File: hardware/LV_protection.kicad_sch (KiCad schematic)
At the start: 4 parts, among them J2 Conn_01x02, Q2 NMOS

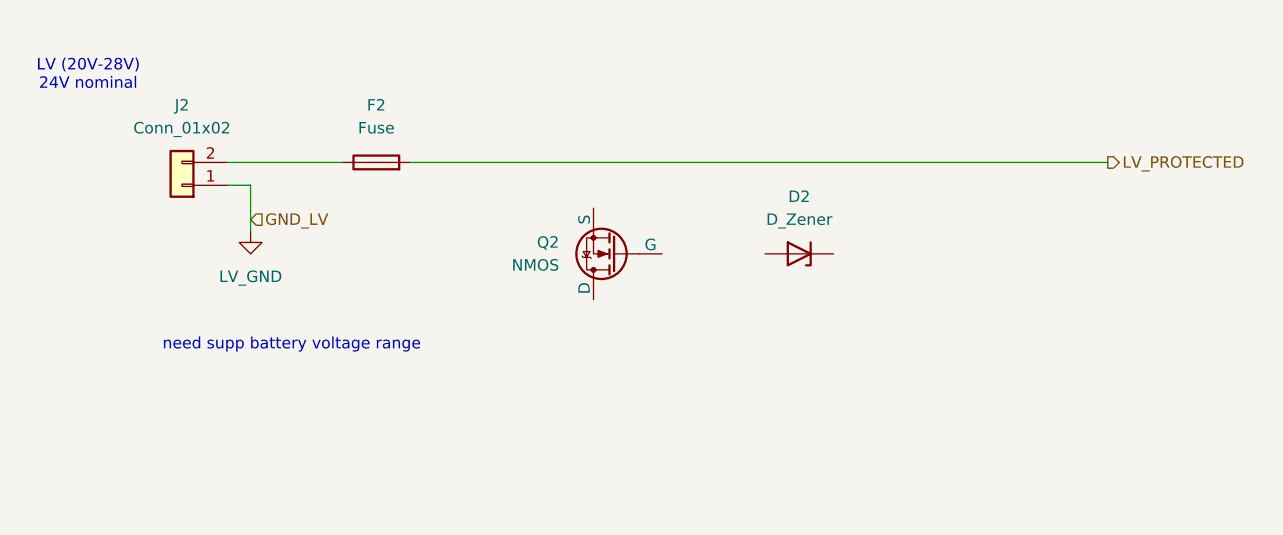
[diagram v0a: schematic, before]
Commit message: did fan circuits, added MCU design block, made buck converter, added VIP sensing + soft start?
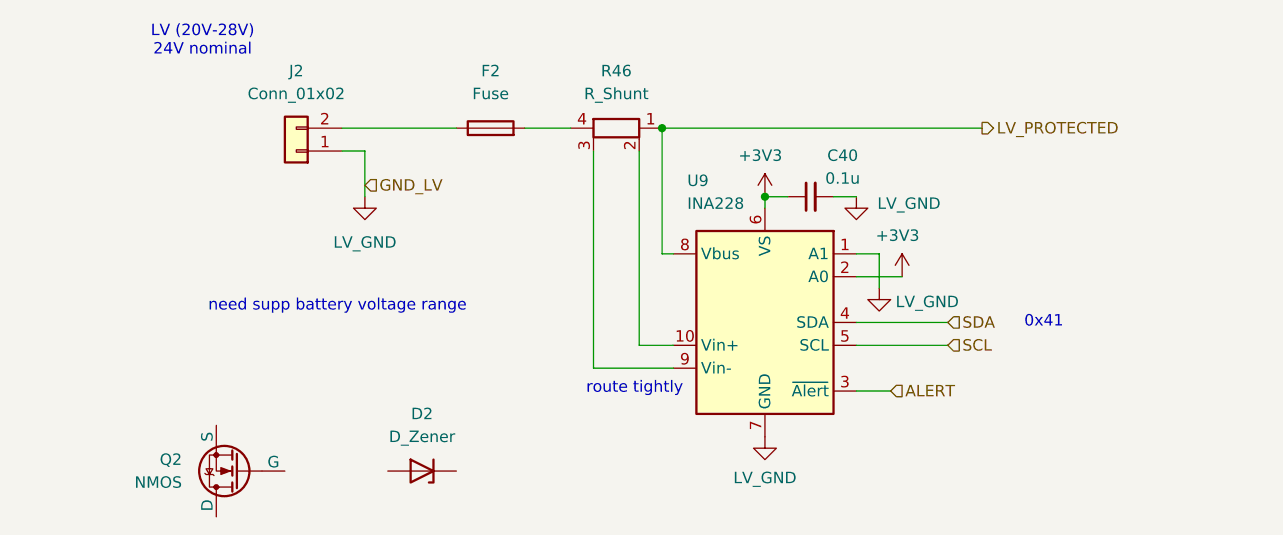
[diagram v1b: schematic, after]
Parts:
- added C40: 0.1u, symbol Device:C_Small
- added R46: R_Shunt, symbol Device:R_Shunt
- added U9: INA228, Package_SO:TSSOP-10_3x3mm_P0.5mm, symbol Sensor_Energy:INA228
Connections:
- net LV_GND: now also C40.2, U9.1 (A1), U9.7 (GND)
- net LV_PROTECTED: now also R46.1, U9.8 (Vbus); no longer F2.2
- new net: R46.2, U9.10 (Vin+)
- new net: R46.3, U9.9 (Vin-)
- new net: F2.2, R46.4
- new net +3V3: C40.1, U9.2 (A0), U9.6 (VS)
- new net ALERT: U9.3 (~{Alert})
- new net SCL: U9.5 (SCL)
- new net SDA: U9.4 (SDA)
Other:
- note added: "0x41"
- note added: "route tightly"
- moved on the sheet: D2, F2, J2, Q2
